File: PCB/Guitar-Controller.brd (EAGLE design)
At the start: 160 x 100 mm, 33 parts

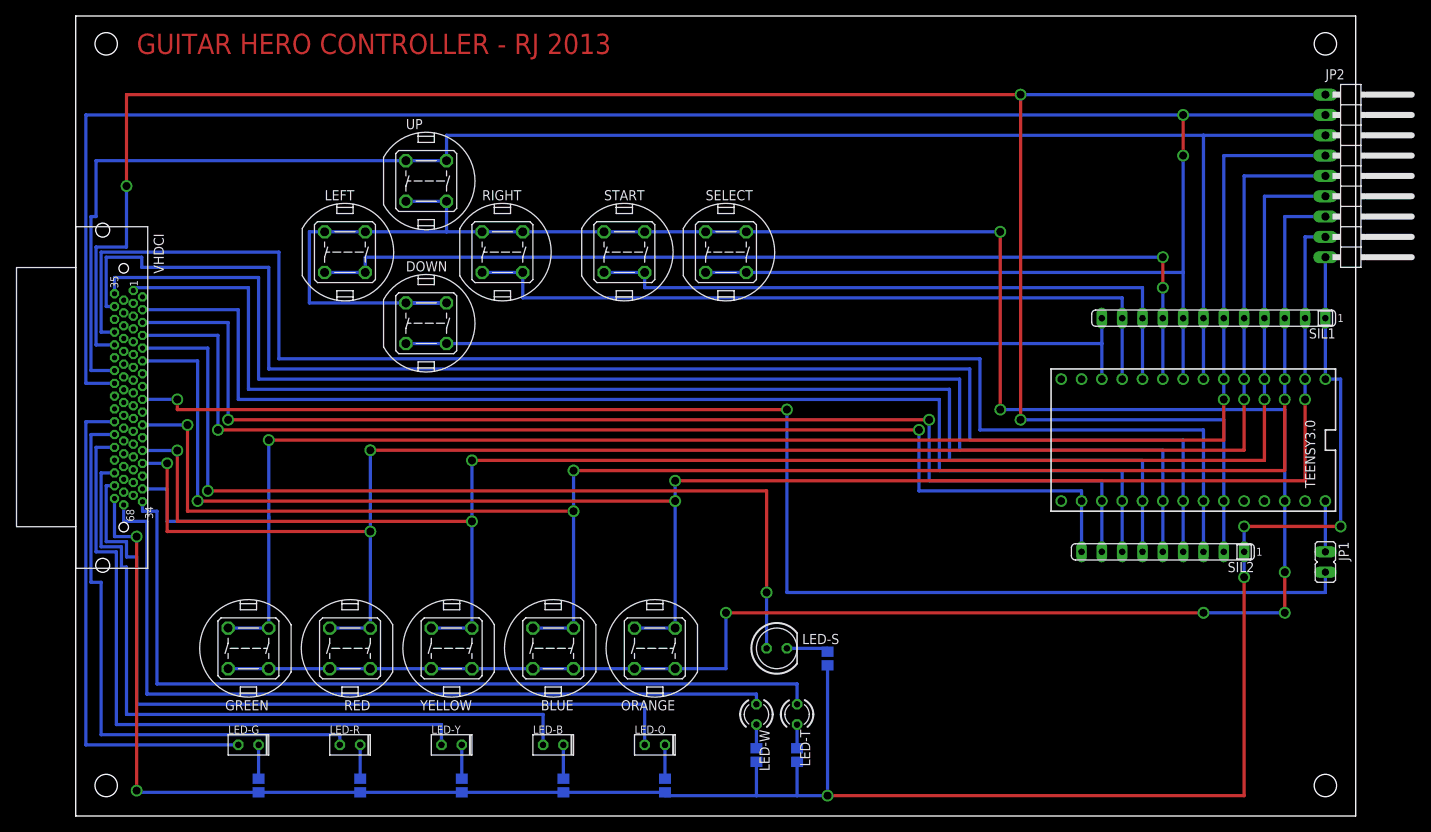
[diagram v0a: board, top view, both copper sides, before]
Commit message: PCB: Final PCB changes (hopefully)
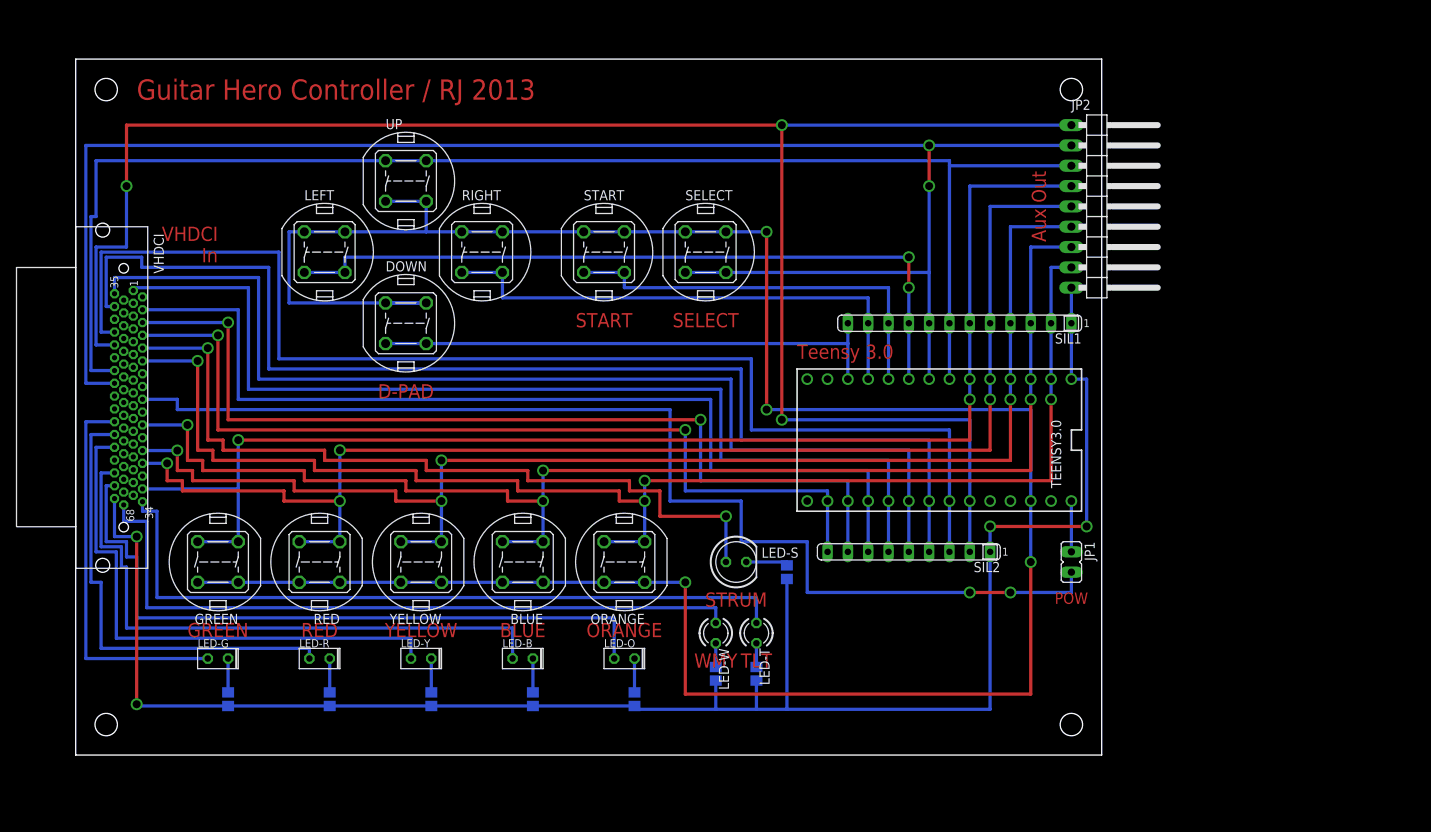
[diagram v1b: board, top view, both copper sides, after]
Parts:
- moved JP2 32.0 mm to (128.3, 76.2)
- moved SIL1 31.8 mm to (110.5, 61.6)
- moved JP1 31.8 mm to (124.5, 31.8)
- moved SIL2 31.7 mm to (104.1, 33.0)
- moved TEENSY3.0 31.7 mm to (108.0, 47.0)
- moved LED-S 11.9 mm to (82.5, 31.8)
- moved R6 11.9 mm to (88.9, 30.5)
- moved ORANGE 11.4 mm to (68.6, 31.8)
- moved YELLOW 11.4 mm to (43.2, 31.8)
- moved BLUE 11.4 mm to (55.9, 31.8)
- moved GREEN 11.4 mm to (17.8, 31.8)
- moved R2 11.4 mm to (31.8, 14.6)
- moved R4 11.4 mm to (57.1, 14.6)
- moved R5 11.4 mm to (69.8, 14.6)
- moved RED 11.4 mm to (30.5, 31.8)
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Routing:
- net SELECT: track 284.8 -> 216.2 mm
- net GND: track 284.4 -> 226.0 mm, vias 6 -> 4
- net GREEN: track 216.7 -> 165.6 mm
- net RED: track 218.0 -> 167.8 mm
- net YELLOW: track 215.8 -> 166.9 mm
- net BLUE: track 215.2 -> 167.5 mm
- net ORANGE: track 219.4 -> 173.0 mm
- net WHAMMY7: track 269.8 -> 228.5 mm
- net 3V3: track 348.6 -> 308.6 mm, vias 6 -> 4
- net UP: track 217.1 -> 179.0 mm
- net WHAMMY6: track 186.9 -> 155.2 mm
- net WHAMMY5: track 178.7 -> 146.9 mm
- net WHAMMY4: track 166.1 -> 134.3 mm
- net WHAMMY2: track 152.7 -> 121.0 mm
- net WHAMMY1: track 148.6 -> 116.8 mm
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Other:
- board size 160 x 100 mm -> 128.2 x 87 mm
- board text added: "Aux Out"
- board text added: "BLUE"
- board text added: "D-PAD"
- board text added: "GREEN"
- board text added: "Guitar Hero Controller / RJ 2013"
- board text added: "ORANGE"
- board text added: "POW"
- board text added: "RED"
- board text added: "SELECT"
- board text added: "START"
- board text added: "STRUM"
- board text added: "TLT"
- board text added: "Teensy 3.0"
- board text added: "VHDCI In"
- board text added: "WMY"
- board text added: "YELLOW"
- board text removed: "GUITAR HERO CONTROLLER - RJ 2013"
